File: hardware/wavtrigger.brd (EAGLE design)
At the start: 63.5 x 58.4 mm, 113 parts, among them J1 5.5x2.1mm Barrel, J3 USD-SOCKETNEW, J5 M02PTH, J6 M08X2, J7 M08X2, J9 M02PTH, U2 MIC5323-3.3, U4 STM32F405RG, U5 PCM5100, U6 LM4990, Y1 8MHz

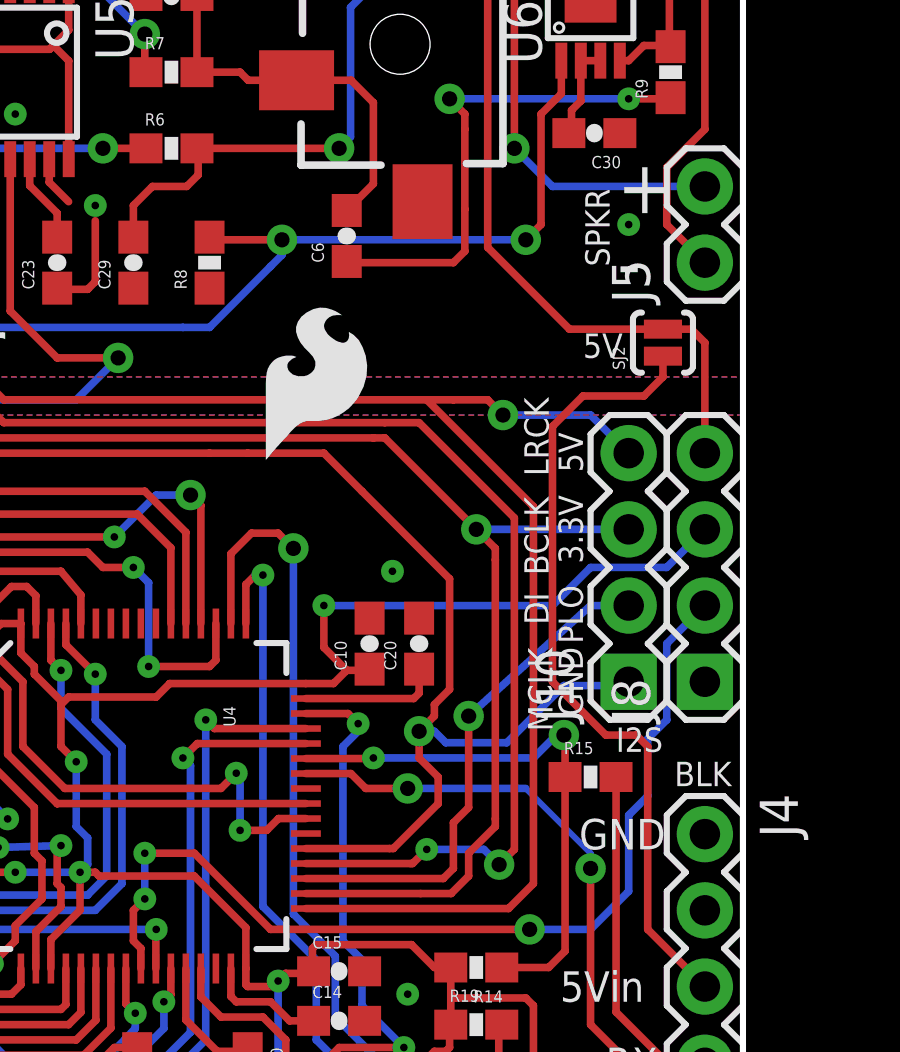
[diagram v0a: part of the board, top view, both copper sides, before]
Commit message: v11 ready for protos
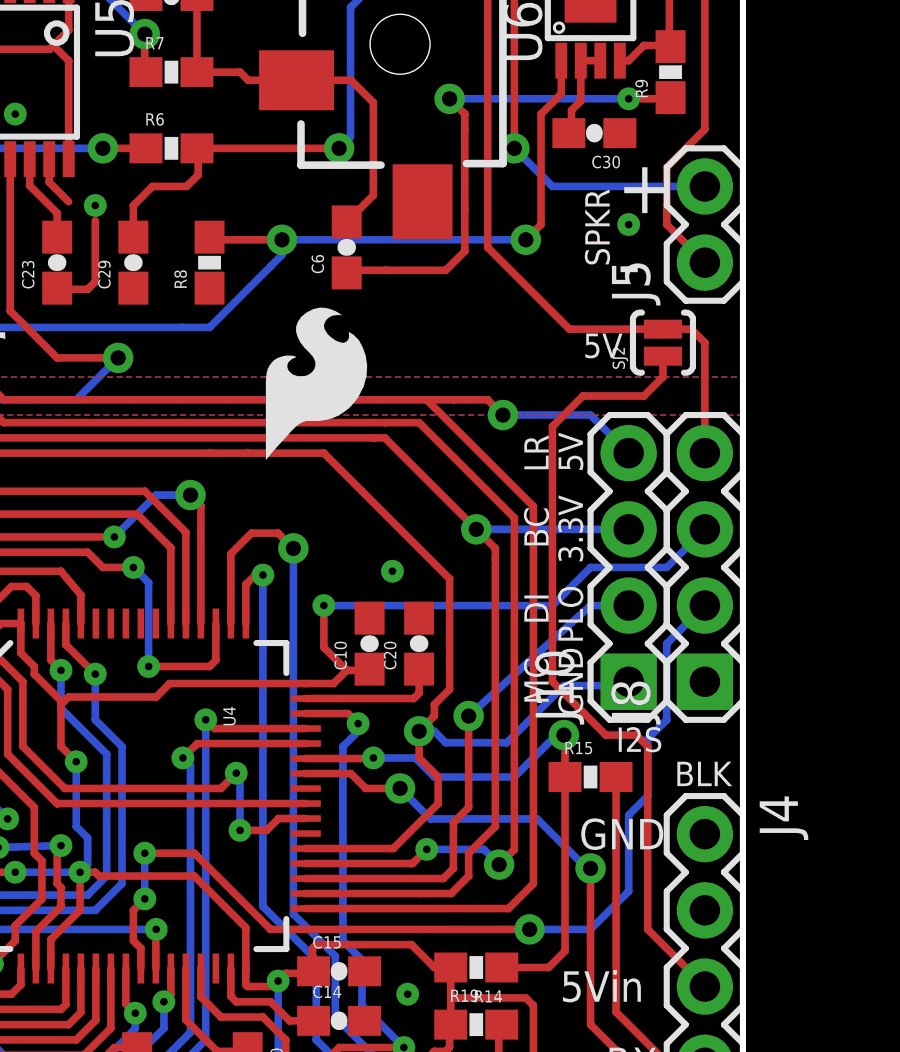
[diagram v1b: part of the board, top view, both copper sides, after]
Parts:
- moved C6 0.38 mm to (50.3, 39.9)
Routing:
- net RXD: track 18.5 -> 19.0 mm
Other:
- board text added: "BC"
- board text added: "LR"
- board text added: "MC"
- board text removed: "BCLK"
- board text removed: "LRCK"
- board text removed: "MCLK"
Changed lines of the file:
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@@
 <circle x="35.941" y="24.638" radius="0" width="0.762" layer="29"/>
 <text x="60.833" y="23.876" size="0.8128" layer="21" font="vector" ratio="15" rot="R180">I2S</text>
-<text x="57.15" y="23.749" size="0.8128" layer="21" font="vector" ratio="15" rot="R90">MCLK</text>
-<text x="57.023" y="28.956" size="0.8128" layer="21" font="vector" ratio="15" rot="R90">BCLK</text>
-<text x="57.023" y="32.258" size="0.8128" layer="21" font="vector" ratio="15" rot="R90">LRCK</text>
+<text x="57.023" y="24.638" size="0.8128" layer="21" font="vector" ratio="15" rot="R90">MC</text>
+<text x="57.023" y="29.845" size="0.8128" layer="21" font="vector" ratio="15" rot="R90">BC</text>
+<text x="57.023" y="32.385" size="0.8128" layer="21" font="vector" ratio="15" rot="R90">LR</text>
 <text x="57.023" y="27.305" size="0.8128" layer="21" font="vector" ratio="15" rot="R90">DI</text>
 </plain>
@@
 <element name="FID1" library="SparkFun-Aesthetics" package="MICRO-FIDUCIAL" value="FIDUCIALUFIDUCIAL" x="1.016" y="52.832"/>
 <element name="FID2" library="SparkFun-Aesthetics" package="MICRO-FIDUCIAL" value="FIDUCIALUFIDUCIAL" x="58.42" y="6.35"/>
-<element name="C6" library="SparkFun-Capacitors" package="0603-CAP" value=".39uF" x="50.292" y="40.259" rot="R90"/>
+<element name="C6" library="SparkFun-Capacitors" package="0603-CAP" value=".39uF" x="50.292" y="39.878" rot="R90"/>
 <element name="TP1" library="SparkFun-Passives" package="TP_15TH" value="TEST-POINTTP_15TH_THRU" x="35.941" y="24.638"/>
 <element name="J10" library="SparkFun-Connectors" package="1X04" value="" x="59.69" y="25.4" rot="R90"/>
@@
 <wire x1="50.435" y1="45.45" x2="51.181" y2="44.704" width="0.254" layer="1"/>
 <wire x1="51.181" y1="44.704" x2="51.181" y2="41.998" width="0.254" layer="1"/>
-<wire x1="51.181" y1="41.998" x2="50.292" y2="41.109" width="0.254" layer="1"/>
+<wire x1="51.181" y1="41.998" x2="51.181" y2="41.617" width="0.254" layer="1"/>
+<wire x1="51.181" y1="41.617" x2="50.292" y2="40.728" width="0.254" layer="1"/>
 </signal>
 <signal name="FILTER">
@@
 <contactref element="U4" pad="42"/>
 <contactref element="J4" pad="5"/>
-<wire x1="50.927" y1="21.844" x2="52.324" y2="21.844" width="0.254" layer="1"/>
-<via x="52.324" y="21.844" extent="1-16" drill="0.508"/>
-<wire x1="52.324" y1="21.844" x2="56.261" y2="21.844" width="0.254" layer="16"/>
+<wire x1="50.927" y1="21.844" x2="52.07" y2="21.844" width="0.254" layer="1"/>
+<via x="52.07" y="21.844" extent="1-16" drill="0.508"/>
 <via x="58.42" y="19.177" extent="1-16" drill="0.508"/>
 <wire x1="58.42" y1="19.177" x2="58.42" y2="13.97" width="0.254" layer="1"/>
 <wire x1="58.42" y1="13.97" x2="62.23" y2="10.16" width="0.254" layer="1"/>
-<wire x1="56.261" y1="21.844" x2="58.42" y2="19.685" width="0.2032" layer="16"/>
-<wire x1="58.42" y1="19.685" x2="58.42" y2="19.177" width="0.2032" layer="16"/>
 <wire x1="50.927" y1="21.844" x2="50.431" y2="22.34" width="0.254" layer="1"/>
 <wire x1="50.431" y1="22.34" x2="48.93" y2="22.34" width="0.254" layer="1"/>
+<wire x1="58.42" y1="19.177" x2="58.293" y2="19.177" width="0.254" layer="16"/>
+<wire x1="58.293" y1="19.177" x2="56.642" y2="20.828" width="0.254" layer="16"/>
+<wire x1="56.642" y1="20.828" x2="53.086" y2="20.828" width="0.254" layer="16"/>
+<wire x1="53.086" y1="20.828" x2="52.07" y2="21.844" width="0.254" layer="16"/>
 </signal>
 <signal name="N$9">
@@
 <wire x1="51.181" y1="22.86" x2="51.161" y2="22.84" width="0.254" layer="1"/>
 <wire x1="51.161" y1="22.84" x2="48.93" y2="22.84" width="0.254" layer="1"/>
-<wire x1="51.181" y1="22.86" x2="56.515" y2="22.86" width="0.254" layer="16"/>
 <wire x1="56.515" y1="22.86" x2="57.277" y2="23.622" width="0.254" layer="16"/>
 <wire x1="57.277" y1="23.622" x2="57.531" y2="23.622" width="0.254" layer="16"/>
+<wire x1="51.181" y1="22.86" x2="52.578" y2="22.86" width="0.254" layer="16"/>
+<wire x1="52.578" y1="22.86" x2="53.213" y2="22.225" width="0.254" layer="16"/>
+<wire x1="53.213" y1="22.225" x2="55.88" y2="22.225" width="0.254" layer="16"/>
+<wire x1="55.88" y1="22.225" x2="56.515" y2="22.86" width="0.254" layer="16"/>
 </signal>
 <signal name="N$7">
@@
 <wire x1="61.048" y1="44.831" x2="61.087" y2="44.87" width="0.254" layer="1"/>
 <wire x1="54.229" y1="41.148" x2="54.229" y2="39.751" width="0.254" layer="1"/>
-<wire x1="54.229" y1="39.751" x2="53.848" y2="39.37" width="0.254" layer="1"/>
-<wire x1="53.848" y1="39.37" x2="50.331" y2="39.37" width="0.254" layer="1"/>
-<wire x1="50.331" y1="39.37" x2="50.292" y2="39.409" width="0.254" layer="1"/>
+<wire x1="54.229" y1="39.751" x2="53.594" y2="39.116" width="0.254" layer="1"/>
+<wire x1="53.594" y1="39.116" x2="51.601" y2="39.116" width="0.254" layer="1"/>
 <wire x1="54.229" y1="43.815" x2="54.229" y2="44.323" width="0.254" layer="1"/>
 <wire x1="54.229" y1="44.323" x2="53.721" y2="44.831" width="0.254" layer="1"/>
+<wire x1="51.601" y1="39.116" x2="50.38" y2="39.116" width="0.254" layer="1"/>
+<wire x1="50.38" y1="39.116" x2="50.292" y2="39.028" width="0.254" layer="1"/>
 </signal>
 <signal name="N$22">
